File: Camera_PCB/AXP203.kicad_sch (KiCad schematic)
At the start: 39 parts, among them J3 USB_C_Receptacle_PowerOnly_6P, SW1 PWR, SW2 RST, U1 AXP203

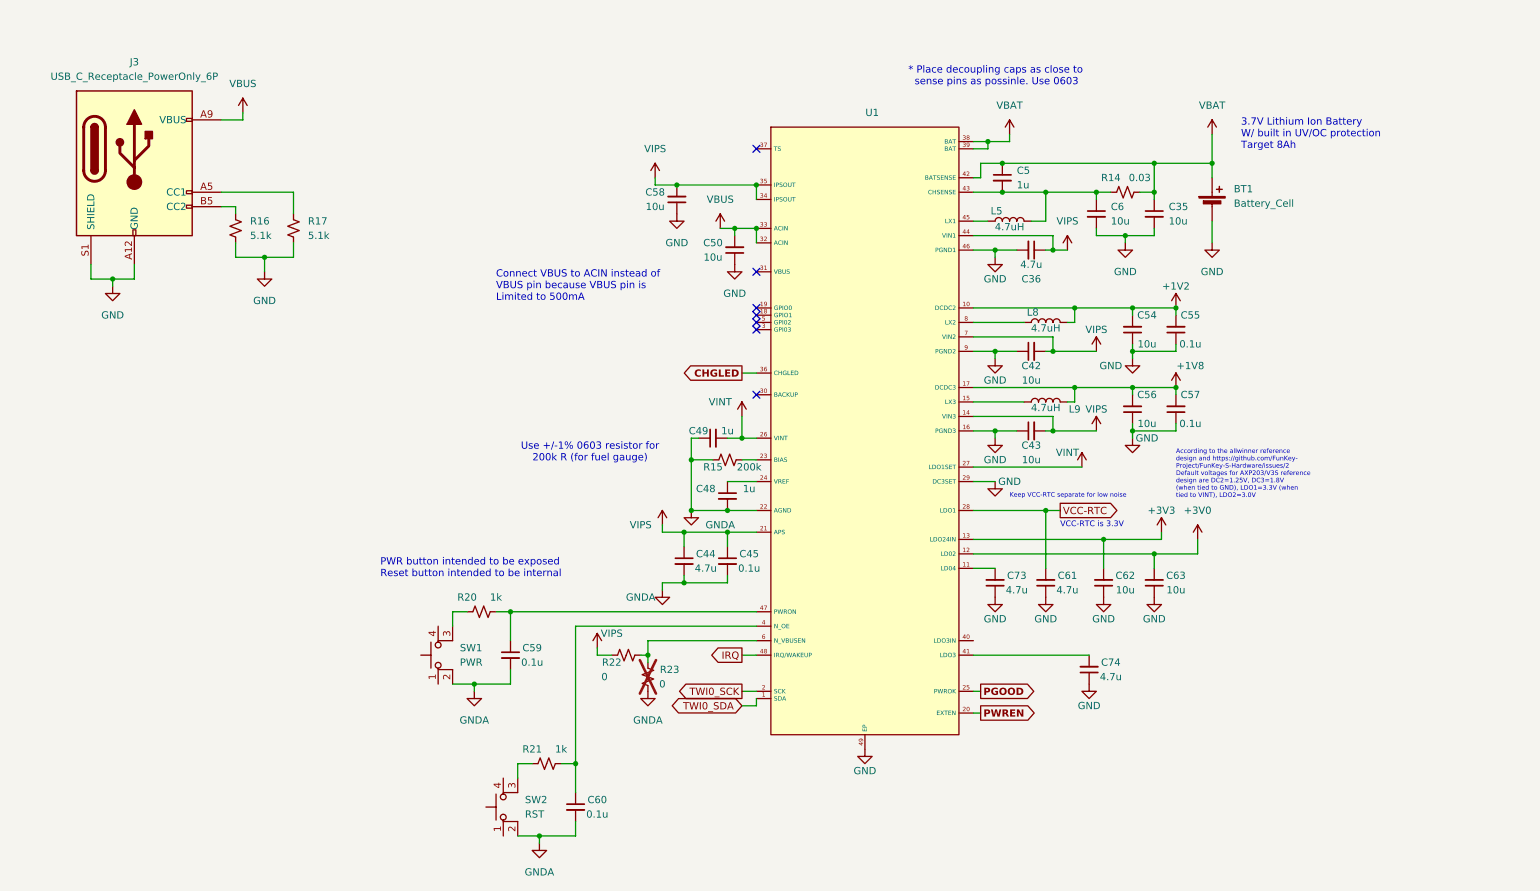
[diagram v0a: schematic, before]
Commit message: cleaned up Camera_PCB \repository
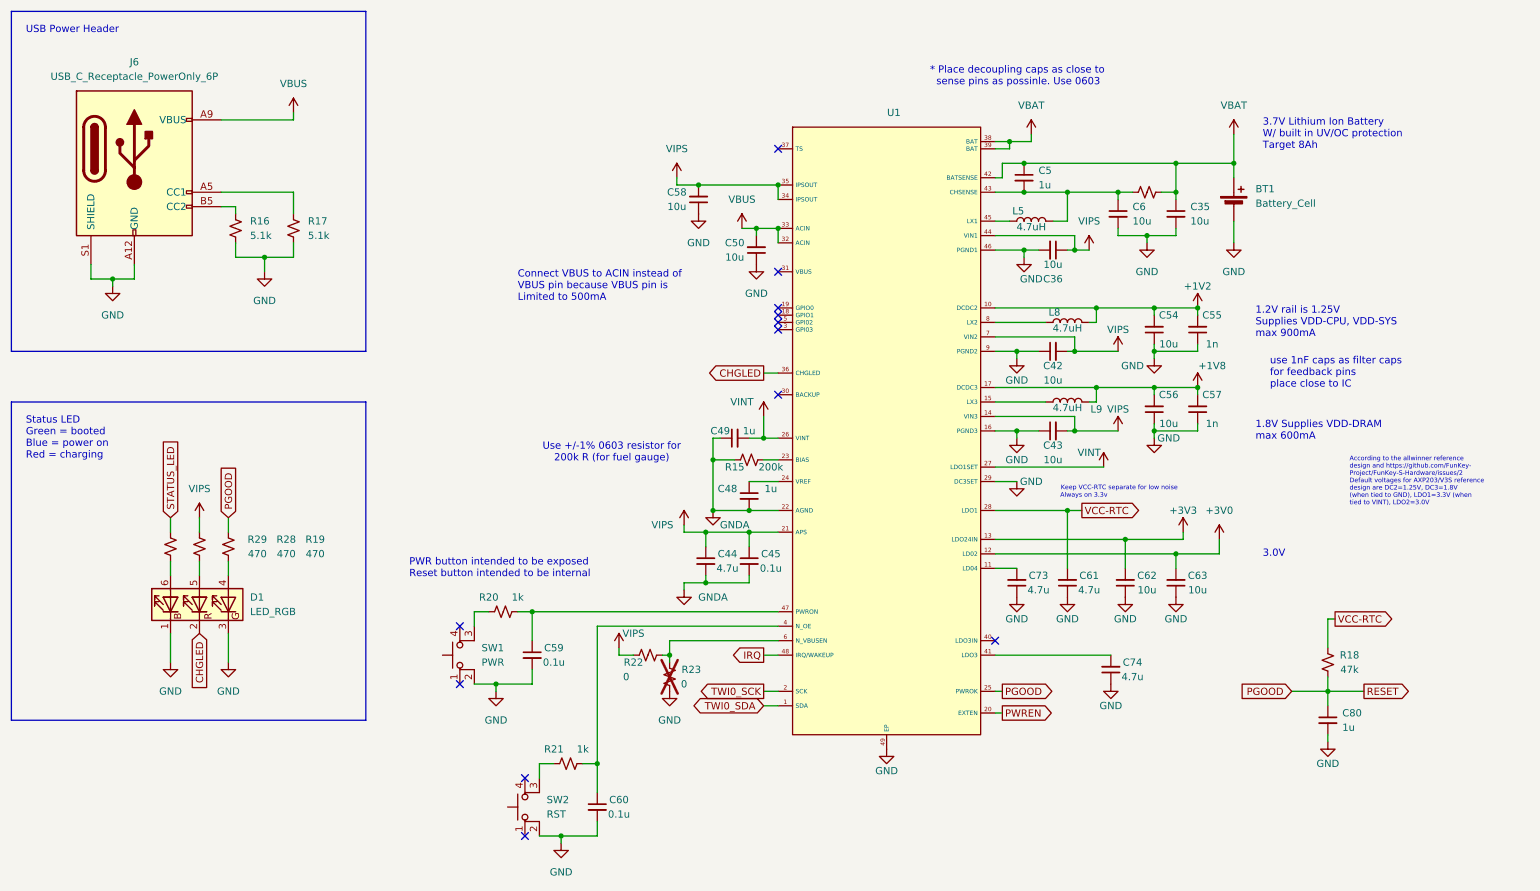
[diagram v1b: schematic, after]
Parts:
- added C80: 1u, Capacitor_SMD:C_0603_1608Metric_Pad1.08x0.95mm_HandSolder, symbol Device:C_Small
- added D1: LED_RGB, BackupCamCustomParts:RGB_LED IN-S66TFT5R5G5B, symbol Device:LED_RGB
- added R18: 47k, Resistor_SMD:R_0603_1608Metric_Pad0.98x0.95mm_HandSolder, symbol Device:R_Small_US
- added R19, R28, R29: 470, Resistor_SMD:R_0603_1608Metric_Pad0.98x0.95mm_HandSolder, symbol Device:R_Small_US
- C35, C42, C43, C50, C54, C56, C58, C6, C62, C63: footprint (none) -> Capacitor_SMD:C_0805_2012Metric_Pad1.18x1.45mm_HandSolder; DPN (none) -> GRM21BZ71E106KE15L; Distributor (none) -> DigiKey
- C36: value 4.7u -> 10u; footprint (none) -> Capacitor_SMD:C_0805_2012Metric_Pad1.18x1.45mm_HandSolder; DPN (none) -> GRM21BZ71E106KE15L; Distributor (none) -> DigiKey
- C44, C61, C73, C74: footprint (none) -> Capacitor_SMD:C_0805_2012Metric_Pad1.18x1.45mm_HandSolder; DPN (none) -> GRM21BZ71H475ME15K; Distributor (none) -> DigiKey
- C45, C59, C60: footprint (none) -> Capacitor_SMD:C_0603_1608Metric_Pad1.08x0.95mm_HandSolder; DPN (none) -> GRM188R72A104KA35D; Distributor (none) -> DigiKey
- C48, C49, C5: footprint (none) -> Capacitor_SMD:C_0603_1608Metric_Pad1.08x0.95mm_HandSolder; DPN (none) -> GCM188R71E105KA64D; Distributor (none) -> DigiKey
- C55, C57: value 0.1u -> 1n; footprint (none) -> Capacitor_SMD:C_0603_1608Metric_Pad1.08x0.95mm_HandSolder; DPN (none) -> GRM1885C1H102JA01D; Distributor (none) -> DigiKey
- L5, L8, L9: footprint (none) -> Inductor_SMD:L_TDK_SLF6045; DPN (none) -> SLF6045T-4R7N2R4-3PF; Distributor (none) -> DigiKey
- R14: footprint (none) -> Resistor_SMD:R_1206_3216Metric; DPN (none) -> PE1206DRM070R03L; Distributor (none) -> DigiKey
- R15: footprint (none) -> Resistor_SMD:R_0603_1608Metric_Pad0.98x0.95mm_HandSolder; DPN (none) -> RC0603FR-07200KL; Distributor (none) -> DigiKey
- R16, R17: footprint (none) -> Resistor_SMD:R_0603_1608Metric_Pad0.98x0.95mm_HandSolder; DPN (none) -> RC0603FR-075K1L; Distributor (none) -> DigiKey
- R20, R21: footprint (none) -> Resistor_SMD:R_0603_1608Metric_Pad0.98x0.95mm_HandSolder; DPN (none) -> RC0603FR-101KL; Distributor (none) -> DigiKey
- R22, R23: footprint (none) -> Resistor_SMD:R_0603_1608Metric_Pad0.98x0.95mm_HandSolder; DPN (none) -> RC0603JR-070RL; Distributor (none) -> DigiKey
- SW1, SW2: footprint (none) -> Button_Switch_SMD:SW_SPST_PTS647_Sx38; DPN (none) -> Y97KT23B5NAFP; Distributor (none) -> DigiKey
- U1: Distributor (none) -> AliExpress
- renumbered J3 to J6
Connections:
- net CHGLED: now also D1.2 (GK)
- net GND: now also C59.2, C60.2, R23.1, SW1.2, SW2.2, C80.2, D1.1 (RK), D1.3 (BK)
- net GNDA: no longer C59.2, C60.2, R23.1, SW1.2, SW2.2
- net PGOOD: now also C80.1, R18.2, R19.1
- net VCC-RTC: now also R18.1
- net VIPS: now also R28.1
- new net: D1.4 (BA), R19.2
- new net: D1.5 (GA), R28.2
- new net: D1.6 (RA), R29.2
- new net STATUS_LED: R29.1
- no-connect marks 7 -> 12
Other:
- note added: "1.2V rail is 1.25V Supplies VDD-CPU, VDD-SYS max 900mA"
- note added: "1.8V Supplies VDD-DRAM max 600mA"
- note added: "3.0V"
- note added: "Always on 3.3v"
- note added: "Status LED Green = booted Blue = power on Red = charging"
- note added: "USB Power Header"
- note added: "use 1nF caps as filter caps for feedback pins place close to IC"
- note removed: "VCC-RTC is 3.3V"
- moved on the sheet: BT1, C35, C36, C42, C43, C44, C45, C48, C49, C5, C50, C54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
